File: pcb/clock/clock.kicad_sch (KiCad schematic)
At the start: 28 parts, among them J1 Conn_02x05_Odd_Even, Q1 Q_PMOS_GSD, Q2 Q_PMOS_GSD, Q3 Q_PMOS_GSD, Q4 HX2301A, SW1 SW_DIP_x01, SW2 SW_DIP_x01, U1 LSD080BAG-103A-01, U2 LSD080BAG-103A-01, U3 74HC595, U4 LSD080BAG-103A-01, U5 LSD080BAG-103A-01, U6 74HC595

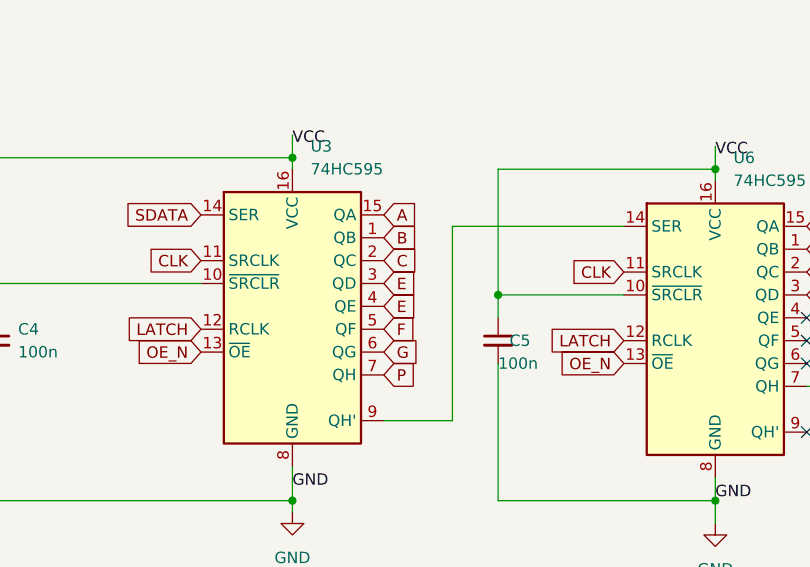
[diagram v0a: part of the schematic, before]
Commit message: first complete pcb of the clock
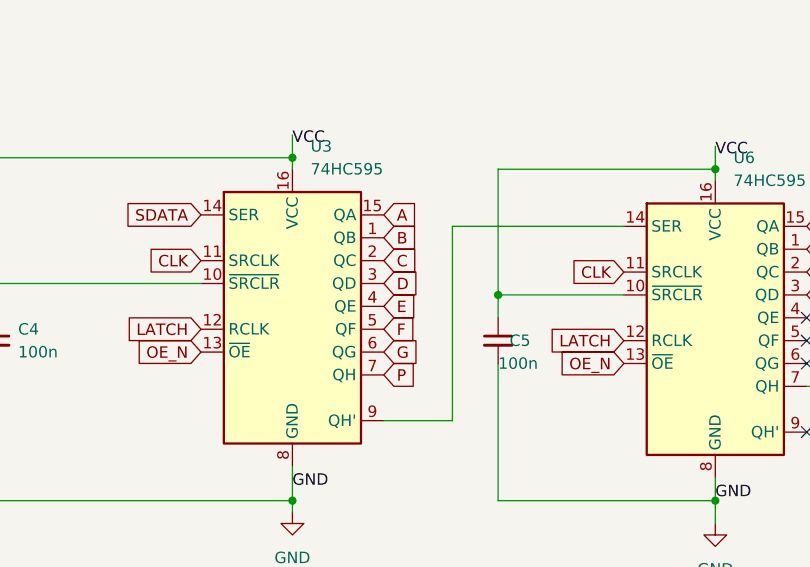
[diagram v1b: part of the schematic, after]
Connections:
- net D: now also U3.3 (QD)
- net E: no longer U3.3 (QD)
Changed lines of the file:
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@@
     )
   )
-  (global_label "E" (shape input) (at 132.08 115.57 0) (fields_autoplaced)
+  (global_label "D" (shape input) (at 132.08 115.57 0) (fields_autoplaced)
     (effects (font (size 1.27 1.27)) (justify left))
-    (property "Intersheet References" "${INTERSHEET_REFS}" (id 0) (at 135.6421 115.4906 0)
+    (property "Intersheet References" "${INTERSHEET_REFS}" (id 0) (at 135.7631 115.4906 0)
       (effects (font (size 1.27 1.27)) (justify left) hide)
     )
